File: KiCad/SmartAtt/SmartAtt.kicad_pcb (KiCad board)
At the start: 2 copper layers, 109.9 x 107.2 mm, 8 parts, among them J16 CON1, J17 CON1, J8 CON1, J9 CON1

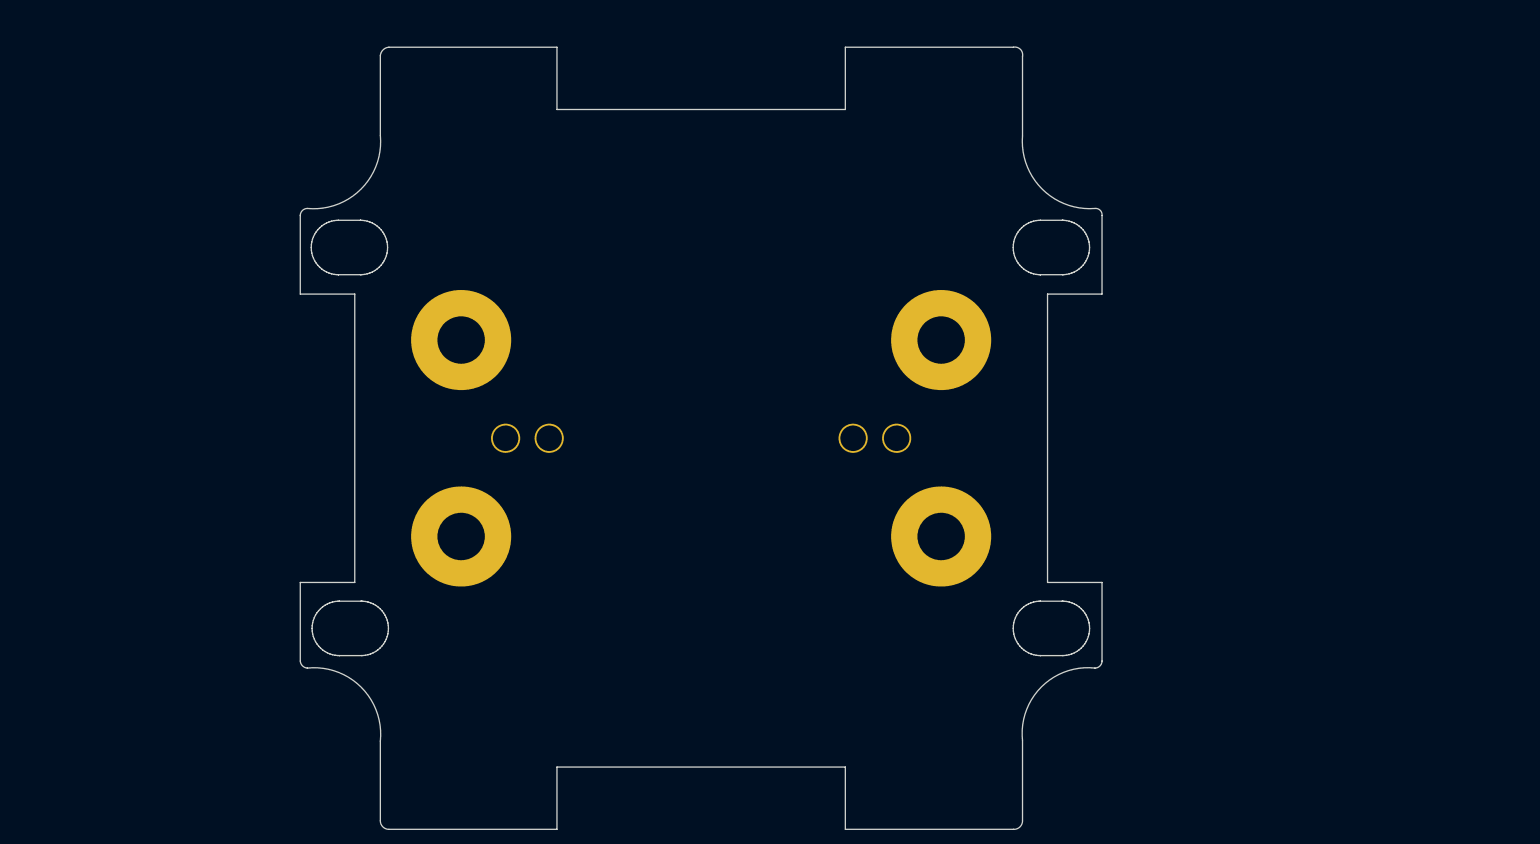
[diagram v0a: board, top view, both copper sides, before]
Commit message: ...
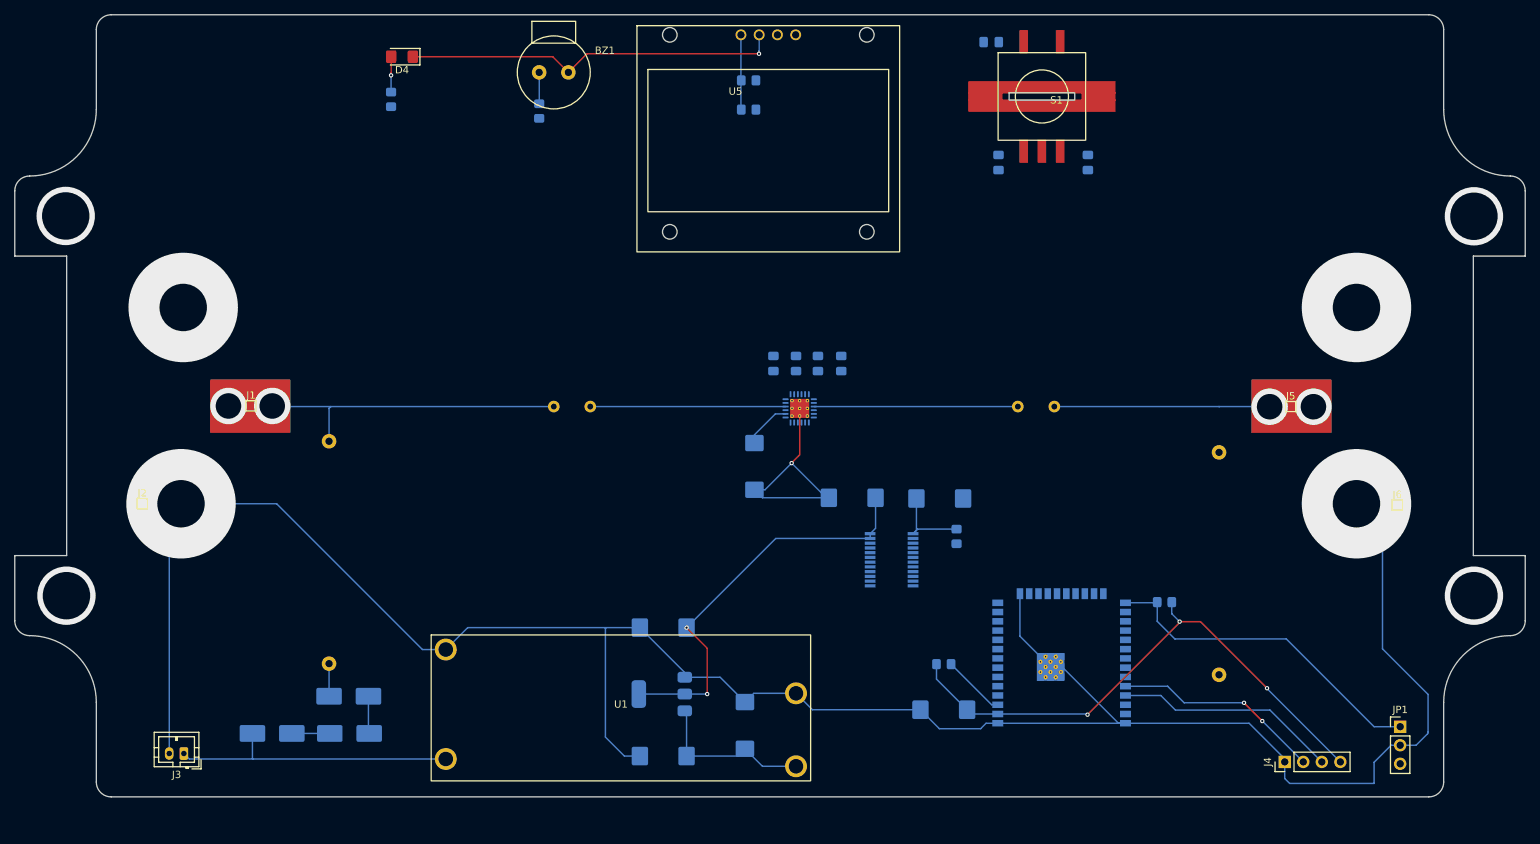
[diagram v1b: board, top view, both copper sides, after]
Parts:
- removed ? (x4): , 
- removed J16, J17, J8, J9: CON1, VIA
- added BZ1: Buzzer, Alexeyj4:HC0903A, F.Cu at (121.8, 44.9)
- added C1: 2,2 нФ, Capacitor_THT:C_Disc_D10.0mm_W2.5mm_P5.00mm, B.Cu at (126.8, 90.7)
- added C10: 330 пФ, Capacitor_SMD:C_0805_2012Metric_Pad1.18x1.45mm_HandSolder, B.Cu at (161.2, 84.8)
- added C11: 47 мкФ, Capacitor_Tantalum_SMD:CP_EIA-7343-31_Kemet-D_Pad2.25x2.55mm_HandSolder, B.Cu at (174.7, 103.3)
- added C12: 100 нФ, Capacitor_SMD:C_0805_2012Metric_Pad1.18x1.45mm_HandSolder, B.Cu at (195.0, 57.2)
- added C13: 47 мкФ, Capacitor_Tantalum_SMD:CP_EIA-7343-31_Kemet-D_Pad2.25x2.55mm_HandSolder, B.Cu at (162.7, 103.2)
- added C14: 100 нФ, Capacitor_SMD:C_0805_2012Metric_Pad1.18x1.45mm_HandSolder, B.Cu at (182.8, 57.2)
- added C15: 100 нФ, Capacitor_SMD:C_0805_2012Metric_Pad1.18x1.45mm_HandSolder, B.Cu at (181.8, 40.8)
- added C16: 2,2 нФ, Capacitor_THT:C_Disc_D10.0mm_W2.5mm_P5.00mm, B.Cu at (190.4, 90.7)
- added C2: 47 мкФ, Capacitor_Tantalum_SMD:CP_EIA-7343-31_Kemet-D_Pad2.25x2.55mm_HandSolder, B.Cu at (136.8, 138.6)
- added C3: 47 мкФ, Capacitor_Tantalum_SMD:CP_EIA-7343-31_Kemet-D_Pad2.25x2.55mm_HandSolder, B.Cu at (136.8, 121.0)
- added C4: 47 мкФ, Capacitor_Tantalum_SMD:CP_EIA-7343-31_Kemet-D_Pad2.25x2.55mm_HandSolder, B.Cu at (148.0, 134.4)
- added C5: 47 мкФ, Capacitor_Tantalum_SMD:CP_EIA-7343-31_Kemet-D_Pad2.25x2.55mm_HandSolder, B.Cu at (175.2, 132.2)
- added C6: 47 мкФ, Capacitor_Tantalum_SMD:CP_EIA-7343-31_Kemet-D_Pad2.25x2.55mm_HandSolder, B.Cu at (149.3, 98.9)
- added C7: 330 пФ, Capacitor_SMD:C_0805_2012Metric_Pad1.18x1.45mm_HandSolder, B.Cu at (151.9, 84.8)
- added C8: 330 пФ, Capacitor_SMD:C_0805_2012Metric_Pad1.18x1.45mm_HandSolder, B.Cu at (155.0, 84.8)
- added C9: 330 пФ, Capacitor_SMD:C_0805_2012Metric_Pad1.18x1.45mm_HandSolder, B.Cu at (158.0, 84.8)
- added D1: 10BQ040, Diode_SMD:D_SMB_Handsoldering, B.Cu at (83.2, 135.5)
- added D2: 10BQ040, Diode_SMD:D_SMB_Handsoldering, B.Cu at (93.8, 135.5)
- added D3: 10BQ040, Diode_SMD:D_SMB_Handsoldering, B.Cu at (93.7, 130.4)
- added D4: LED, LED_SMD:LED_1206_3216Metric_Pad1.42x1.75mm_HandSolder, F.Cu at (101.0, 42.8)
- added IC1: 74LVC4245APW,112, Alexeyj4:SOP65P640X110-24N, B.Cu at (168.1, 111.7)
- added J1: RF_base, TestPoint:TestPoint_Pad_1.0x1.0mm, F.Cu at (80.3, 90.6)
- added J2: RF_base_gnd, TestPoint:TestPoint_Pad_1.0x1.0mm, F.Cu at (65.4, 104.0)
- added J3: 12V, Connector_JST:JST_PH_B2B-PH-K_1x02_P2.00mm_Vertical, F.Cu at (71.1, 138.2)
- added J4: UART_FW, Connector_PinHeader_2.54mm:PinHeader_1x04_P2.54mm_Vertical, F.Cu at (222.0, 139.4)
- added J5: RF_mine, TestPoint:TestPoint_Pad_1.0x1.0mm, F.Cu at (222.8, 90.7)
- added J6: RF_mine_gnd, TestPoint:TestPoint_Pad_1.0x1.0mm, F.Cu at (237.4, 104.2)
- added JP1: FW, Connector_PinHeader_2.54mm:PinHeader_1x03_P2.54mm_Vertical, F.Cu at (237.8, 134.6)
- added L1: 4 мГн мин., Inductor_THT:L_Axial_L24.0mm_D7.1mm_P30.48mm_Horizontal_Vishay_IM-10-28, B.Cu at (91.0, 95.5)
- added L2: 4 мГн мин., Inductor_THT:L_Axial_L24.0mm_D7.1mm_P30.48mm_Horizontal_Vishay_IM-10-28, B.Cu at (213.0, 97.0)
- added R1: 10 кОм, Resistor_SMD:R_0805_2012Metric_Pad1.20x1.40mm_HandSolder, B.Cu at (175.2, 126.0)
- added R2: 10 кОм, Resistor_SMD:R_0805_2012Metric_Pad1.20x1.40mm_HandSolder, B.Cu at (205.5, 117.5)
- added R3: 0 Ом, Resistor_SMD:R_0805_2012Metric_Pad1.20x1.40mm_HandSolder, B.Cu at (148.5, 46.0)
- added R4: 1 кОм, Resistor_SMD:R_0805_2012Metric_Pad1.20x1.40mm_HandSolder, B.Cu at (177.0, 108.5)
- added R5: NU, Resistor_SMD:R_0805_2012Metric_Pad1.20x1.40mm_HandSolder, B.Cu at (148.5, 50.0)
- added R6: 1 кОм, Resistor_SMD:R_0805_2012Metric_Pad1.20x1.40mm_HandSolder, B.Cu at (99.5, 48.6)
- added R7: 100 Ом, Resistor_SMD:R_0805_2012Metric_Pad1.20x1.40mm_HandSolder, B.Cu at (119.8, 50.2)
- added S1: EC11, Alexeyj4:RotaryEncoder EC11 SMD, F.Cu at (188.7, 48.2)
- added U1: MP-N, Alexeyj4:MPN, F.Cu at (131.0, 132.0)
- added U2: AMS1117-3.3, Package_TO_SOT_SMD:SOT-223-3_TabPin2, B.Cu at (136.6, 130.1)
- added U3: ESP32-WROOM-32E, RF_Module:ESP32-WROOM-32D, B.Cu at (191.4, 125.9)
- added U4: HMC542BLP4ETR, Package_DFN_QFN:QFN-24-1EP_4x4mm_P0.5mm_EP2.6x2.6mm_ThermalVias, B.Cu at (155.5, 91.0)
- added U5: OLED, Alexeyj4:OLED I2C, F.Cu at (151.2, 53.5)
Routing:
- net GND: track 0.00 -> 397.1 mm, vias 0 -> 4
- net +3.3V: track 0.00 -> 131.6 mm, vias 0 -> 5
- net Net-(JP1-A): track 0.00 -> 46.3 mm
- net Net-(J1-Pin_1): track 0.00 -> 43.5 mm, vias 0 -> 2
- net Net-(D1-K): track 0.00 -> 39.7 mm
- net +5V: track 0.00 -> 33.9 mm
- net /TX0: track 0.00 -> 30.7 mm
- net Net-(J5-Pin_1): track 0.00 -> 29.6 mm, vias 0 -> 2
- net /RX0: track 0.00 -> 28.7 mm, vias 0 -> 2
- net Net-(U4-RF2): track 0.00 -> 28.0 mm
- net Net-(U4-RF1): track 0.00 -> 26.8 mm
- net (no net): track 11.1 -> 0.00 mm, vias 0 -> 6
- net Net-(U5-VCC): track 0.00 -> 10.3 mm
- net Net-(U3-EN): track 0.00 -> 8.71 mm
- net Net-(U4-Vcc): track 0.00 -> 6.58 mm
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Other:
- board size 109.9 x 107.2 mm -> 207 x 107.2 mm
